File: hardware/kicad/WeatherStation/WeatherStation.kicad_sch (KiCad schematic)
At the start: 0 parts

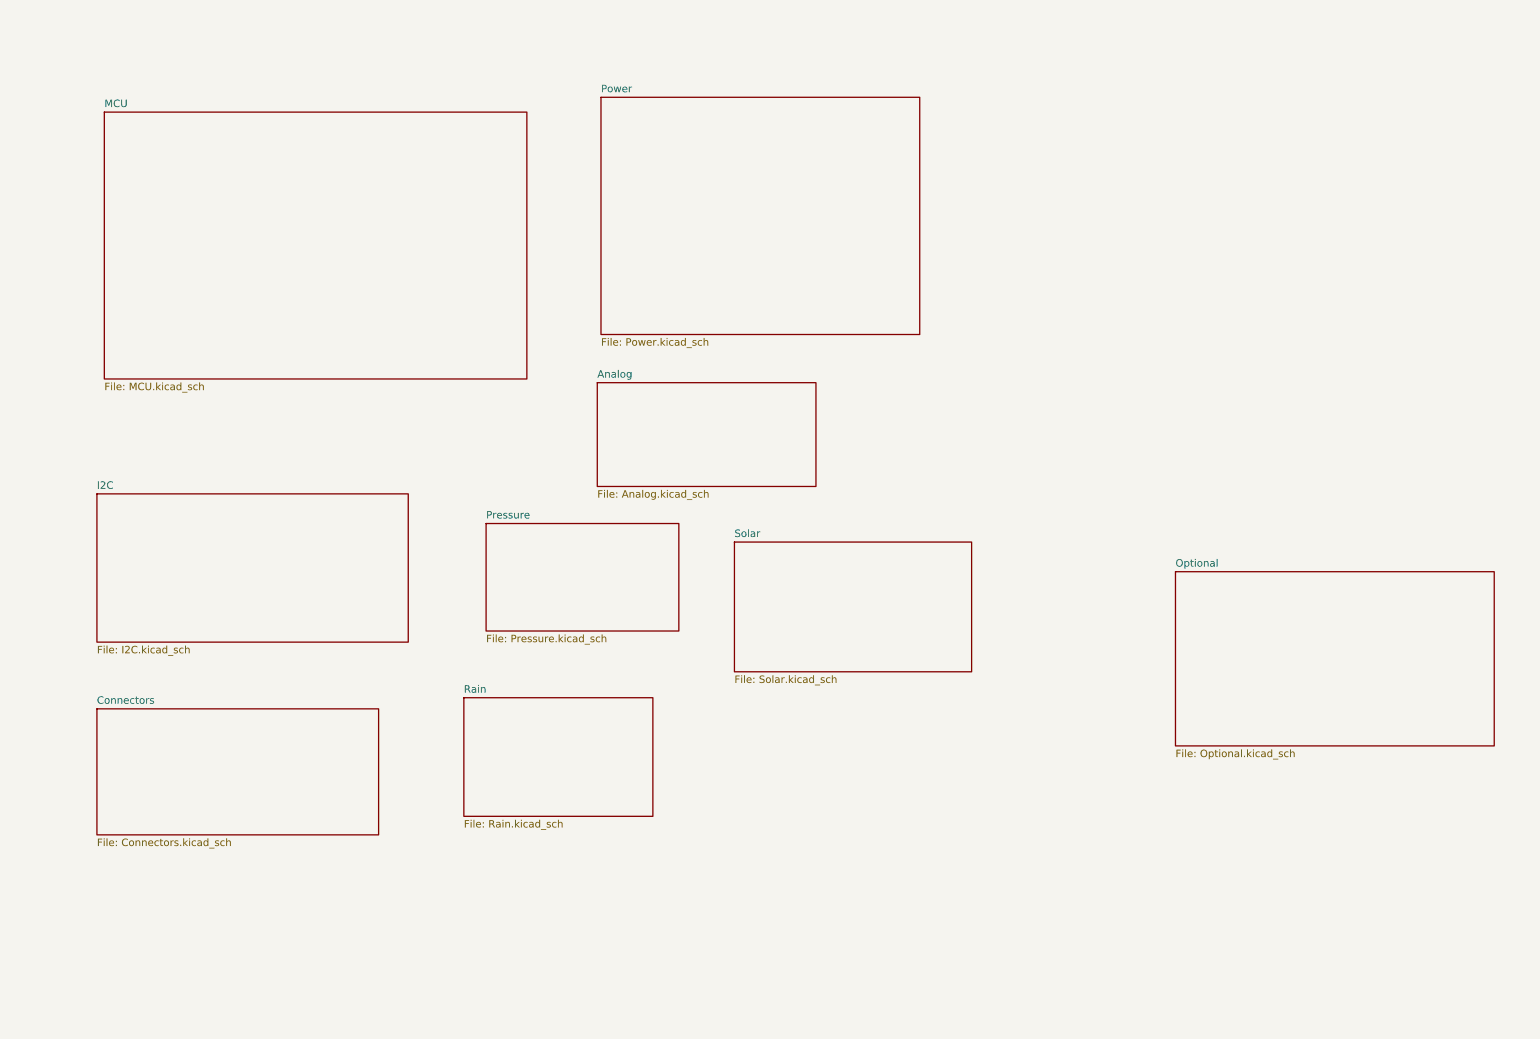
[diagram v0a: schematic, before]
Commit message: Chages to Hardware - not yet finished
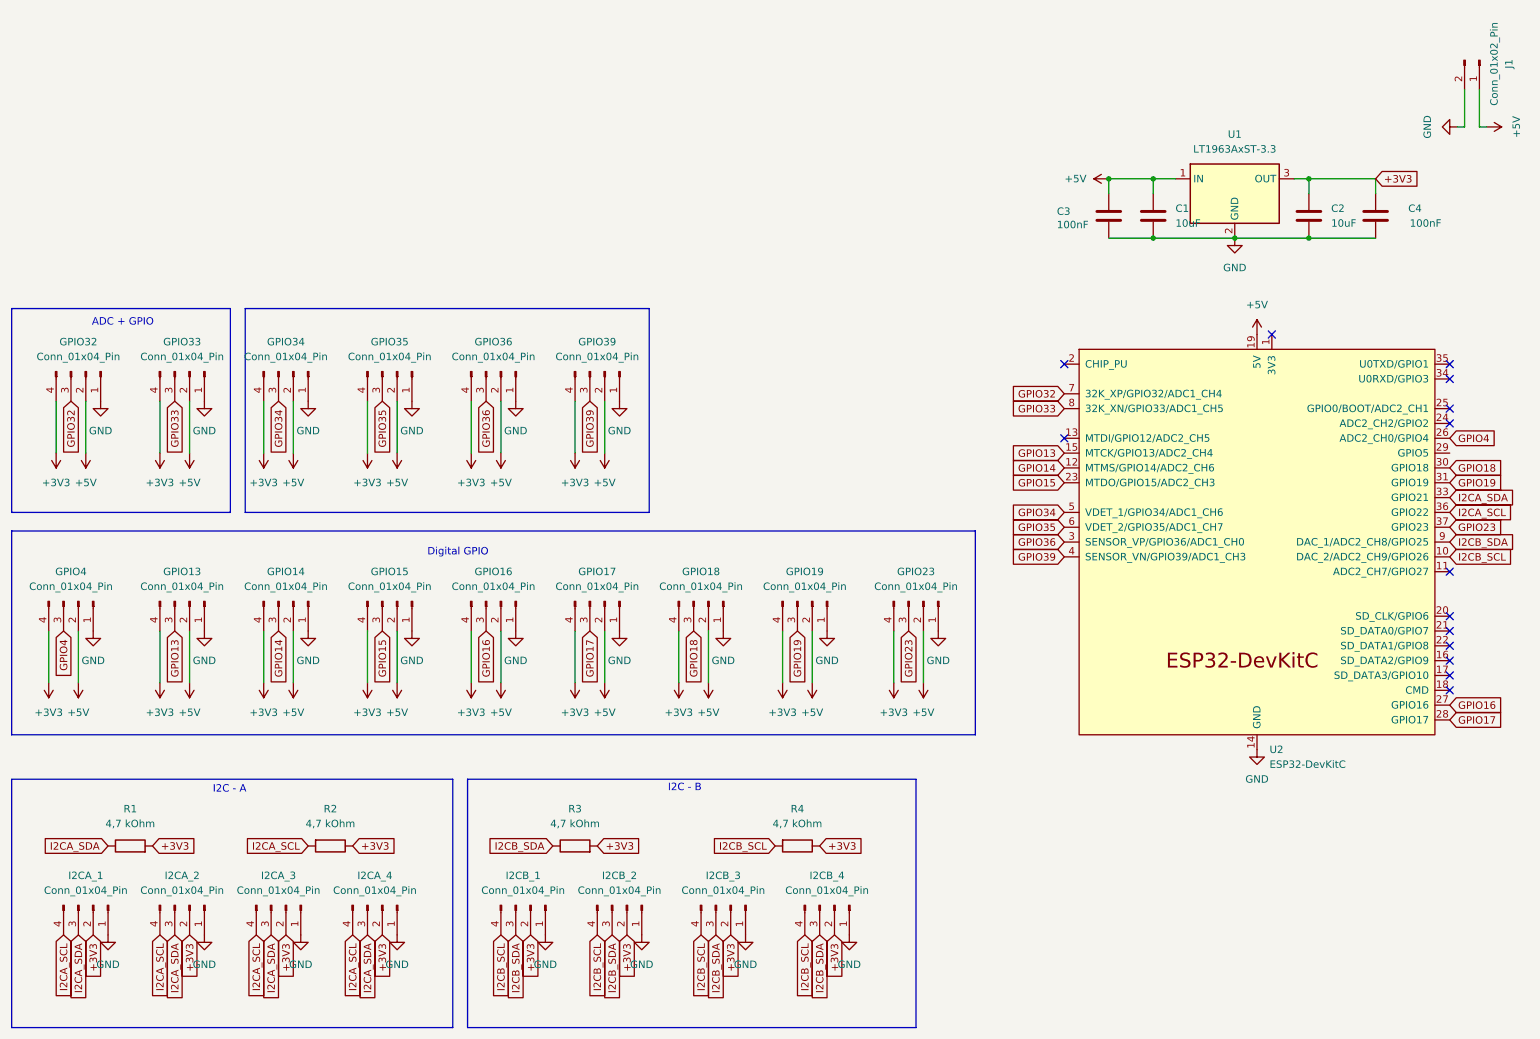
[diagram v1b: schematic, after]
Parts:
- added C1, C2: 10uF, Capacitor_SMD:C_1206_3216Metric_Pad1.33x1.80mm_HandSolder, symbol Device:C
- added C3, C4: 100nF, Capacitor_SMD:C_1206_3216Metric_Pad1.33x1.80mm_HandSolder, symbol Device:C
- added GPIO13, GPIO14, GPIO15, GPIO16, GPIO17, GPIO18, GPIO19, GPIO23, GPIO32, GPIO33, GPIO34, GPIO35, GPIO36, GPIO39, GPIO4: Conn_01x04_Pin, Connector_JST:JST_PH_B4B-PH-K_1x04_P2.00mm_Vertical, symbol Connector:Conn_01x04_Pin
- added I2CA_1, I2CA_2, I2CA_3, I2CB_1, I2CB_2, I2CB_3: Conn_01x04_Pin, Connector_JST:JST_SH_SM04B-SRSS-TB_1x04-1MP_P1.00mm_Horizontal, symbol Connector:Conn_01x04_Pin
- added I2CA_4, I2CB_4: Conn_01x04_Pin, EnvNode:QWIIC_PinSocket_1x04_P2.54mm_Vertical, symbol Connector:Conn_01x04_Pin
- added J1: Conn_01x02_Pin, Connector_JST:JST_PH_B2B-PH-K_1x02_P2.00mm_Vertical, symbol Connector:Conn_01x02_Pin
- added R1, R2, R3, R4: 4,7 kOhm, Resistor_SMD:R_1206_3216Metric_Pad1.30x1.75mm_HandSolder, symbol Device:R
- added U1: LT1963AxST-3.3, Package_TO_SOT_SMD:SOT-223-3_TabPin2, symbol Regulator_Linear:LT1963AxST-3.3
- added U2: ESP32-DevKitC, PCM_Espressif:ESP32-DevKitC, symbol PCM_Espressif:ESP32-DevKitC
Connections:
- new net +3V3: C2.1, C4.2, GPIO13.4 (Pin_4), GPIO14.4 (Pin_4), GPIO15.4 (Pin_4), GPIO16.4 (Pin_4), GPIO17.4 (Pin_4), GPIO18.4 (Pin_4), GPIO19.4 (Pin_4), GPIO23.4 (Pin_4), GPIO32.4 (Pin_4), GPIO33.4 (Pin_4), GPIO34.4 (Pin_4), GPIO35.4 (Pin_4), GPIO36.4 (Pin_4), GPIO39.4 (Pin_4), GPIO4.4 (Pin_4), I2CA_1.2 (Pin_2), I2CA_2.2 (Pin_2), I2CA_3.2 (Pin_2), I2CA_4.2 (Pin_2), I2CB_1.2 (Pin_2), I2CB_2.2 (Pin_2), I2CB_3.2 (Pin_2), I2CB_4.2 (Pin_2), R1.2, R2.1, R3.2, R4.1, U1.3 (OUT)
- new net +5V: C1.1, C3.2, GPIO13.2 (Pin_2), GPIO14.2 (Pin_2), GPIO15.2 (Pin_2), GPIO16.2 (Pin_2), GPIO17.2 (Pin_2), GPIO18.2 (Pin_2), GPIO19.2 (Pin_2), GPIO23.2 (Pin_2), GPIO32.2 (Pin_2), GPIO33.2 (Pin_2), GPIO34.2 (Pin_2), GPIO35.2 (Pin_2), GPIO36.2 (Pin_2), GPIO39.2 (Pin_2), GPIO4.2 (Pin_2), J1.1 (Pin_1), U1.1 (IN), U2.19 (5V)
- new net GND: C1.2, C2.2, C3.1, C4.1, GPIO13.1 (Pin_1), GPIO14.1 (Pin_1), GPIO15.1 (Pin_1), GPIO16.1 (Pin_1), GPIO17.1 (Pin_1), GPIO18.1 (Pin_1), GPIO19.1 (Pin_1), GPIO23.1 (Pin_1), GPIO32.1 (Pin_1), GPIO33.1 (Pin_1), GPIO34.1 (Pin_1), GPIO35.1 (Pin_1), GPIO36.1 (Pin_1), GPIO39.1 (Pin_1), GPIO4.1 (Pin_1), I2CA_1.1 (Pin_1), I2CA_2.1 (Pin_1), I2CA_3.1 (Pin_1), I2CA_4.1 (Pin_1), I2CB_1.1 (Pin_1), I2CB_2.1 (Pin_1), I2CB_3.1 (Pin_1), I2CB_4.1 (Pin_1), J1.2 (Pin_2), U1.2 (GND), U2.14 (GND), U2.32 (GND), U2.38 (GND)
- new net GPIO13: GPIO13.3 (Pin_3), U2.15 (MTCK/GPIO13/ADC2_CH4)
- new net GPIO14: GPIO14.3 (Pin_3), U2.12 (MTMS/GPIO14/ADC2_CH6)
- new net GPIO15: GPIO15.3 (Pin_3), U2.23 (MTDO/GPIO15/ADC2_CH3)
- new net GPIO16: GPIO16.3 (Pin_3), U2.27 (GPIO16)
- new net GPIO17: GPIO17.3 (Pin_3), U2.28 (GPIO17)
- new net GPIO18: GPIO18.3 (Pin_3), U2.30 (GPIO18)
- new net GPIO19: GPIO19.3 (Pin_3), U2.31 (GPIO19)
- new net GPIO23: GPIO23.3 (Pin_3), U2.37 (GPIO23)
- new net GPIO32: GPIO32.3 (Pin_3), U2.7 (32K_XP/GPIO32/ADC1_CH4)
- new net GPIO33: GPIO33.3 (Pin_3), U2.8 (32K_XN/GPIO33/ADC1_CH5)
- new net GPIO34: GPIO34.3 (Pin_3), U2.5 (VDET_1/GPIO34/ADC1_CH6)
- new net GPIO35: GPIO35.3 (Pin_3), U2.6 (VDET_2/GPIO35/ADC1_CH7)
- new net GPIO36: GPIO36.3 (Pin_3), U2.3 (SENSOR_VP/GPIO36/ADC1_CH0)
- new net GPIO39: GPIO39.3 (Pin_3), U2.4 (SENSOR_VN/GPIO39/ADC1_CH3)
- new net GPIO4: GPIO4.3 (Pin_3), U2.26 (ADC2_CH0/GPIO4)
- new net I2CA_SCL: I2CA_1.4 (Pin_4), I2CA_2.4 (Pin_4), I2CA_3.4 (Pin_4), I2CA_4.4 (Pin_4), R2.2, U2.36 (GPIO22)
- new net I2CA_SDA: I2CA_1.3 (Pin_3), I2CA_2.3 (Pin_3), I2CA_3.3 (Pin_3), I2CA_4.3 (Pin_3), R1.1, U2.33 (GPIO21)
- new net I2CB_SCL: I2CB_1.4 (Pin_4), I2CB_2.4 (Pin_4), I2CB_3.4 (Pin_4), I2CB_4.4 (Pin_4), R4.2, U2.10 (DAC_2/ADC2_CH9/GPIO26)
- new net I2CB_SDA: I2CB_1.3 (Pin_3), I2CB_2.3 (Pin_3), I2CB_3.3 (Pin_3), I2CB_4.3 (Pin_3), R3.1, U2.9 (DAC_1/ADC2_CH8/GPIO25)
- no-connect marks 0 -> 14
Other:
- removed sheet Analog
- removed sheet Connectors
- removed sheet I2C
- removed sheet MCU
- removed sheet Optional
- removed sheet Power
- removed sheet Pressure
- removed sheet Rain
- removed sheet Solar
- note added: "ADC + GPIO"
- note added: "Digital GPIO"
- note added: "I2C - A"
- note added: "I2C - B"
